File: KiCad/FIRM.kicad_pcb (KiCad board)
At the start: 4 copper layers, 57.5 x 70.3 mm, 95 parts, among them J1 Conn_01x02_Pin, J2 DM3CS-SF, J5 USB_C_Receptacle_USB2.0_16P, Q2 IRLML6402, SW1 PTS815, U1 STM32F405RGTx, U2 MIC5219-3.3YM5, U7 W25Q128JVS, X2 32.768khz, Y1 12 MHz

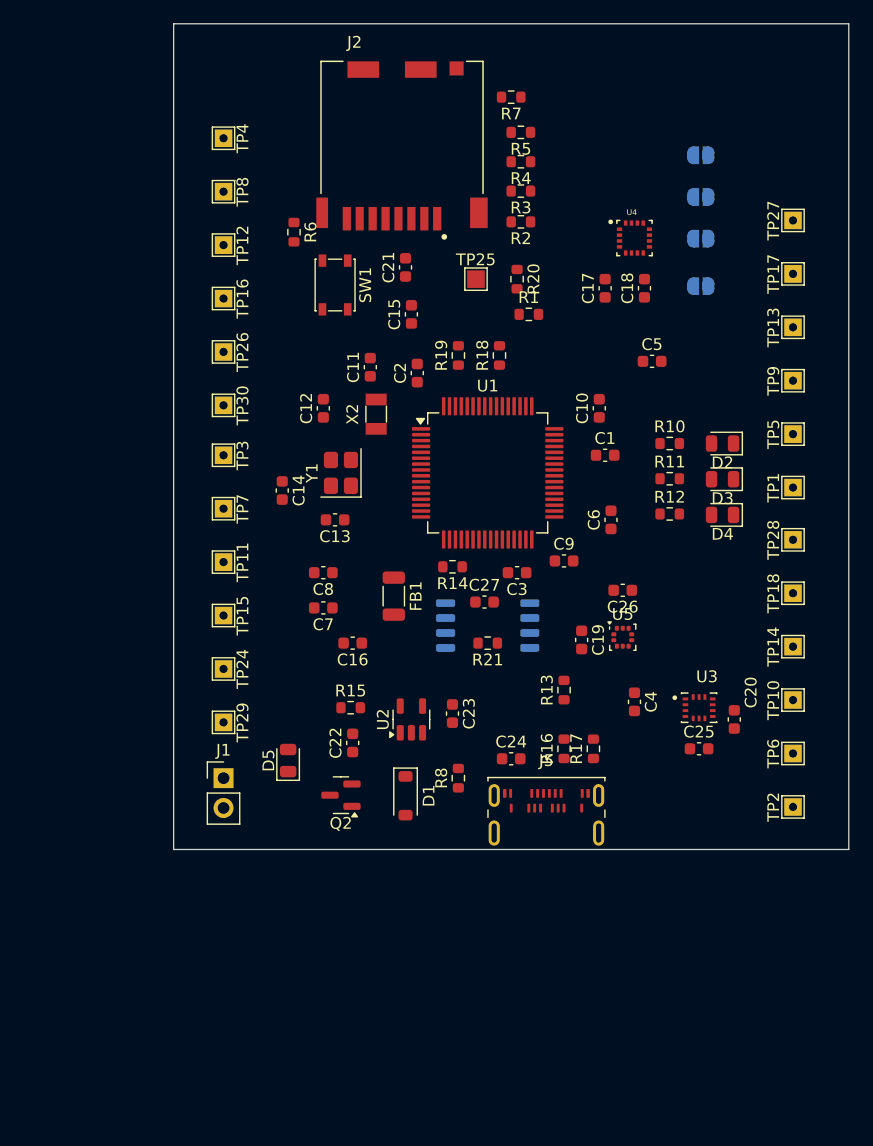
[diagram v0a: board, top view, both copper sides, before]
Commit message: im firm
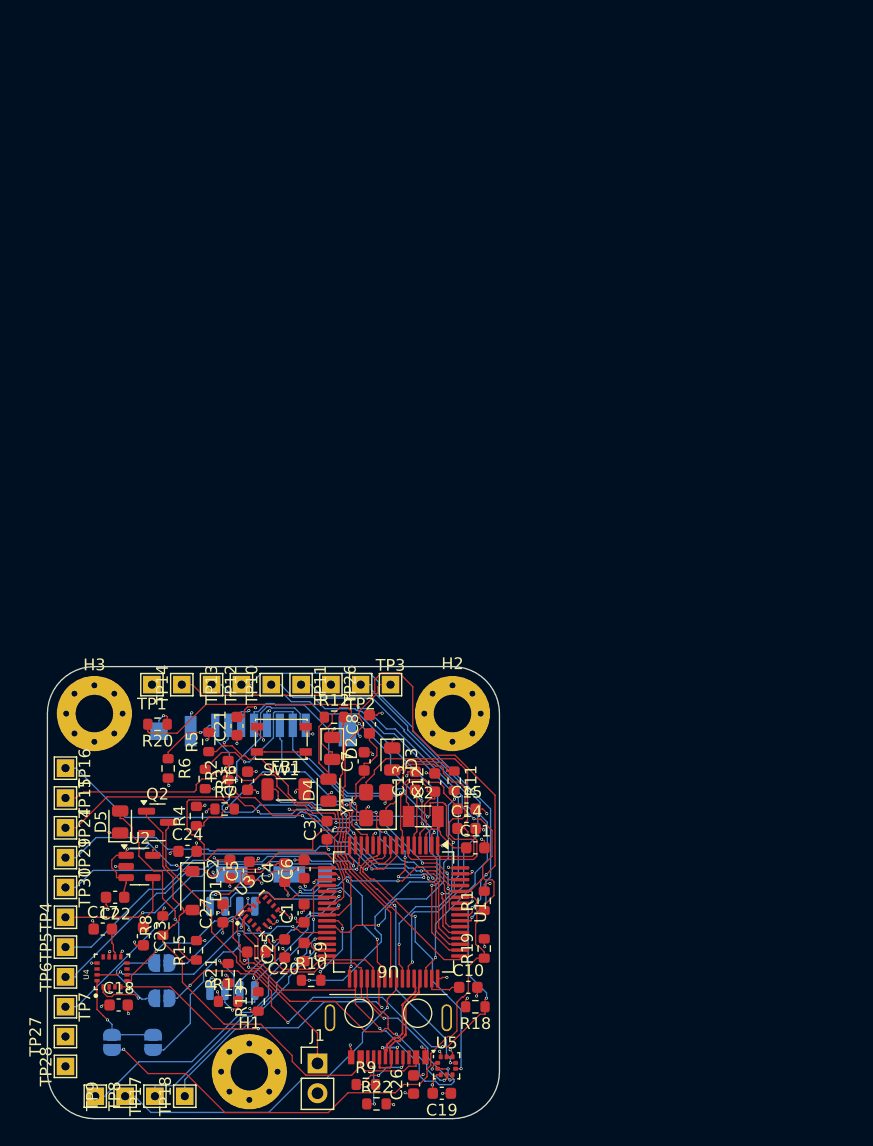
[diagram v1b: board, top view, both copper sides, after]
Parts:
- removed J5: USB_C_Receptacle_USB2.0_16P, Connector_USB:USB_C_Receptacle_Amphenol_124019772112A
- removed R16, R17: 5.1k, Resistor_SMD:R_0603_1608Metric
- added H1: MountingHole_Pad, MountingHole:MountingHole_3.2mm_M3_Pad_Via, F.Cu at (113.2, 130.5)
- added H2: MountingHole_Pad, MountingHole:MountingHole_3.2mm_M3_Pad_Via, F.Cu at (130.5, 100.0)
- added H3: MountingHole_Pad, MountingHole:MountingHole_3.2mm_M3_Pad_Via, F.Cu at (100.0, 100.0)
- added R22: 5.1k, Resistor_SMD:R_0603_1608Metric, F.Cu at (124.0, 133.2)
- added R9: 5.1k, Resistor_SMD:R_0603_1608Metric, F.Cu at (123.1, 131.6)
- added U6: A-USBC-20F0-EA-GSR05, connectors:A-USBC-20F0-EA-GSR05, F.Cu at (125.0, 125.5)
- J2, TP25: moved to B.Cu
- moved TP27 93.1 mm to (97.5, 127.5)
- moved TP17 88.6 mm to (105.2, 132.6)
- moved TP9 83.4 mm to (102.6, 132.6)
- moved JP2 82.8 mm to (105.0, 128.0), turned to -90 degrees
- moved JP4 82.7 mm to (105.8, 121.2)
- moved JP3 82.2 mm to (105.8, 124.2)
- moved JP1 81.6 mm to (101.5, 128.0), turned to -90 degrees
- moved TP8 77.8 mm to (100.1, 132.6)
- moved U4 76.7 mm to (101.5, 122.0), turned to 90 degrees
- moved TP28 76.5 mm to (97.5, 130.0)
- moved TP5 75.8 mm to (97.5, 119.9)
- moved C18 75.7 mm to (102.1, 124.8), turned to 0 degrees
- moved C17 69.4 mm to (100.7, 118.4), turned to 0 degrees
- moved TP4 67.7 mm to (97.5, 117.3), turned to 90 degrees
- moved TP18 67.2 mm to (107.7, 132.6)
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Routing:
- net GND: track 0.00 -> 60.7 mm, vias 0 -> 55
- net /I2C1_SDA: track 0.00 -> 49.9 mm, vias 0 -> 1
- net /PB4: track 0.00 -> 47.0 mm, vias 0 -> 2
- net /BOOT0: track 0.00 -> 46.8 mm, vias 0 -> 2
- net /I2C1_SCL: track 0.00 -> 45.8 mm, vias 0 -> 5
- net /MOSI2: track 0.00 -> 45.6 mm, vias 0 -> 4
- net VBUS: track 0.00 -> 44.7 mm
- net /PB5: track 0.00 -> 42.8 mm, vias 0 -> 4
- net /MISO2: track 0.00 -> 41.9 mm, vias 0 -> 4
- net Net-(D2-A): track 0.00 -> 41.3 mm, vias 0 -> 4
- net /SDIO_D2: track 0.00 -> 41.0 mm, vias 0 -> 3
- net /SDIO_D1: track 0.00 -> 40.5 mm, vias 0 -> 2
- net /SCK2: track 0.00 -> 40.5 mm, vias 0 -> 3
- net /SDIO_D3: track 0.00 -> 39.4 mm, vias 0 -> 4
- net /SDIO_CMD: track 0.00 -> 39.3 mm, vias 0 -> 6
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- added copper zone on In2.Cu, net +3.3V
- added copper zone on In1.Cu, net GND
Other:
- board size 57.5 x 70.3 mm -> 38.5 x 38.5 mm
